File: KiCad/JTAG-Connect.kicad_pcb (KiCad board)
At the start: 2 copper layers, 16.5 x 21 mm, 2 parts, among them J1 Conn_02x05_Odd_Even, J2 Conn_02x03_Odd_Even

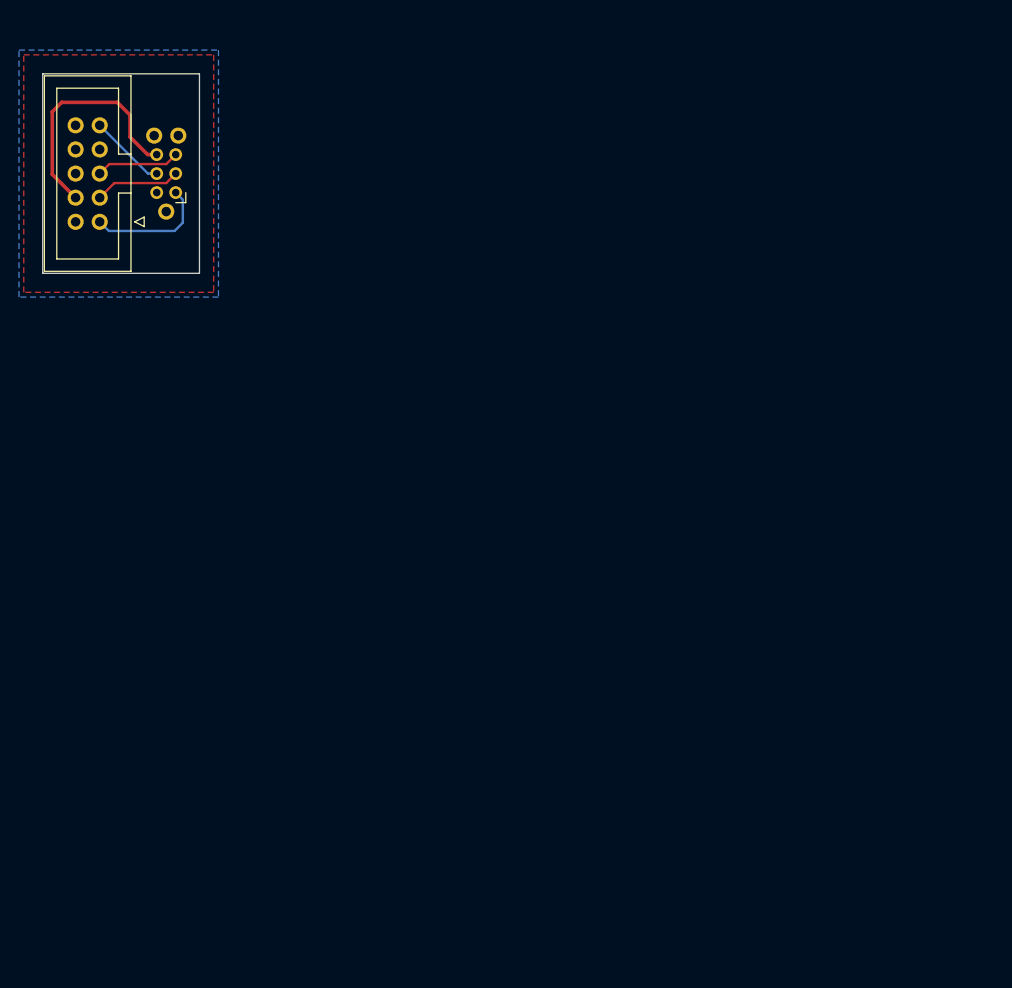
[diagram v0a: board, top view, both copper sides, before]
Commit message: updated design
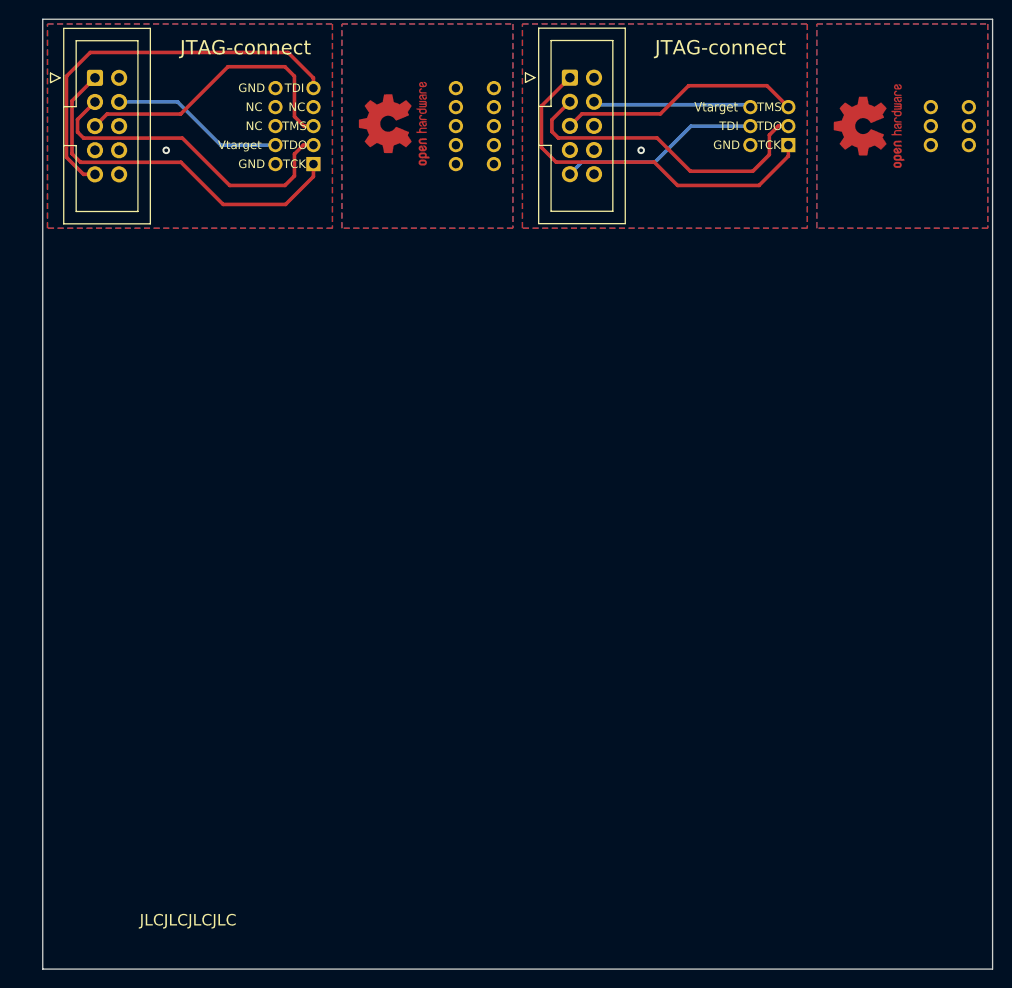
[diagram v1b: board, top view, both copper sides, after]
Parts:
- added J3: Conn_02x05_Odd_Even, JTAG-Connect:PinHeader_2x05_P2.00mm_JTAG_connect_on_SMD_pads, F.Cu at (130.5, 74.0)
- added J4: Conn_02x05_Odd_Even, Connector_IDC:IDC-Header_2x05_P2.54mm_Vertical, F.Cu at (139.5, 64.9)
- added J5: Conn_02x03_Odd_Even, JTAG-Connect:PinHeader_2x03_P2.00mm_JTAG_connect_on_SMD_pads, F.Cu at (161.5, 72.0)
- added J6: Conn_02x03_Odd_Even, JTAG-Connect:PinHeader_2x03_P2.00mm_JTAG_connect_on_SMD_pads, F.Cu at (180.5, 72.0)
- added REF**: OSHW-Logo2_9.8x8mm_Copper, Symbol:OSHW-Logo2_9.8x8mm_Copper, F.Cu at (171.0, 70.0)
- added REF**: OSHW-Logo2_9.8x8mm_Copper, Symbol:OSHW-Logo2_9.8x8mm_Copper, F.Cu at (121.0, 69.8)
- J2: value Conn_02x03_Odd_Even -> Conn_02x05_Odd_Even; footprint Connector_PinHeader_2.00mm:PinHeader_2x03_P2.00mm_Vertical -> JTAG-Connect:PinHeader_2x05_P2.00mm_JTAG_connect_on_SMD_pads
- moved J1 15.2 mm to (89.5, 64.9), turned to 0 degrees
- moved J2 13.8 mm to (111.5, 74.0)
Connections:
- J2 pad 4: TDI -> Vtarget
- J2 pad 6: Vtarget -> Net-(J2-Pad6)
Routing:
- net TCK2: track 0.00 -> 38.7 mm
- net TDO2: track 0.00 -> 33.7 mm
- net TDI: track 8.10 -> 41.5 mm
- net TCK: track 13.0 -> 39.1 mm
- net TMS2: track 0.00 -> 25.7 mm
- net TDO: track 9.05 -> 34.2 mm
- net TMS: track 8.83 -> 30.7 mm
- net TDI2: track 0.00 -> 21.1 mm
- net Vtarget2: track 0.00 -> 16.7 mm
- net Vtarget: track 25.1 -> 18.3 mm
- net GND: vias 0 -> 2
- added copper zone on B.Cu, net (none)
- added copper zone on F.Cu, net (none)
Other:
- board size 16.5 x 21 mm -> 100 x 100 mm
- board text added: "GND"
- board text added: "JLCJLCJLCJLC"
- board text added: "JTAG-connect"
- board text added: "NC"
- board text added: "TCK"
- board text added: "TDI"
- board text added: "TDO"
- board text added: "TMS"
- board text added: "V-CUT"
- board text added: "Vtarget"
